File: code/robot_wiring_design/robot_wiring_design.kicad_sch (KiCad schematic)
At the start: 26 parts, among them J1 Conn_02x20_Counter_Clockwise

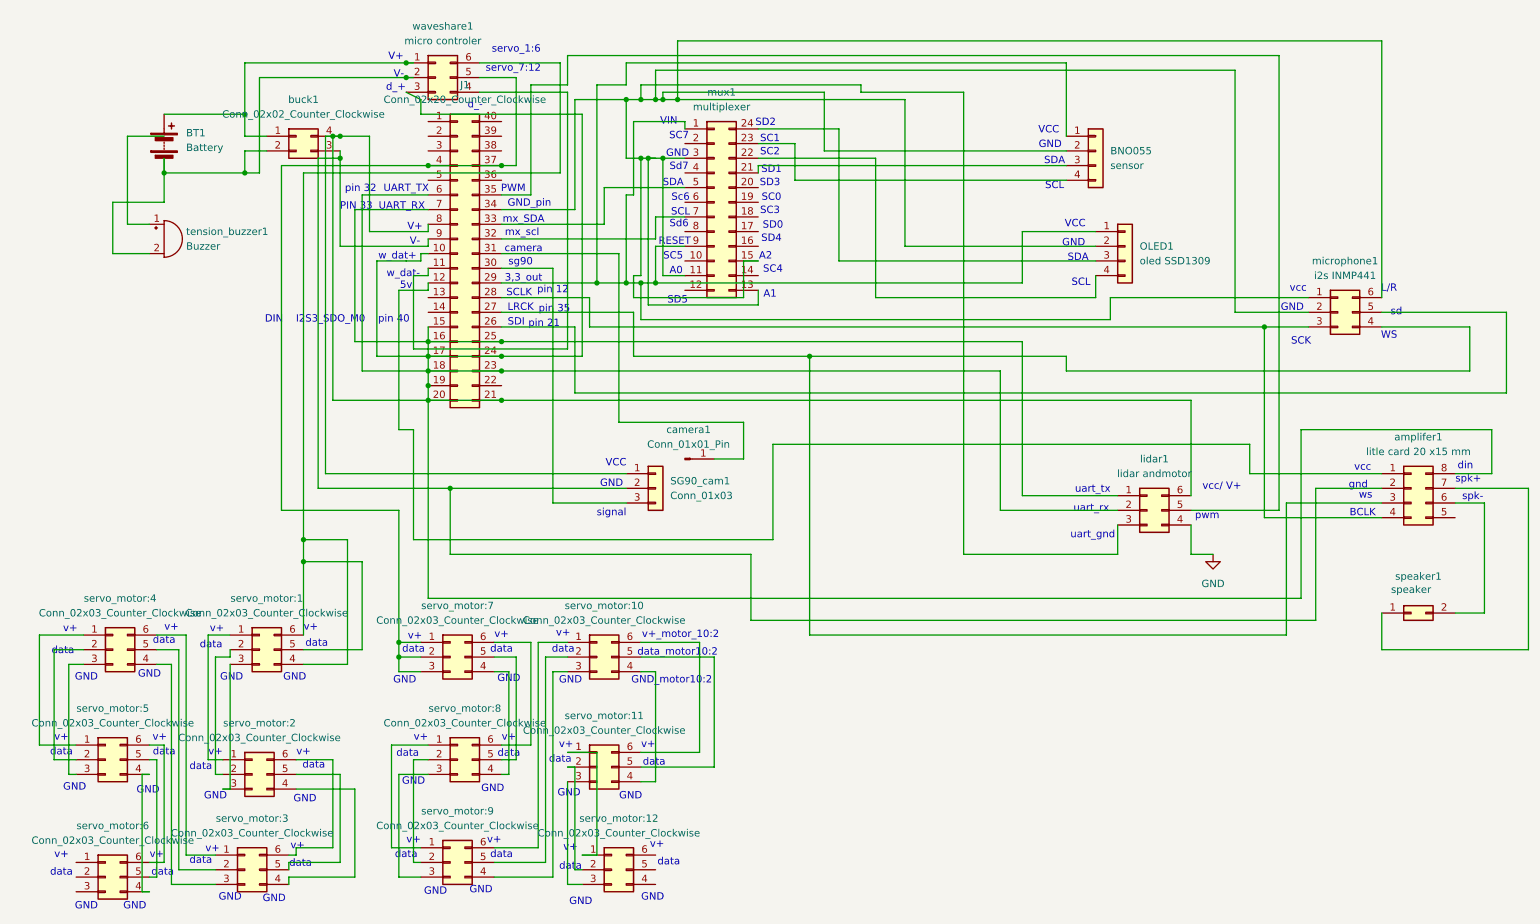
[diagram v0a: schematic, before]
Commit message: add the final pcb update the bom with lesspriced lidar add the new model of the 3d robot design
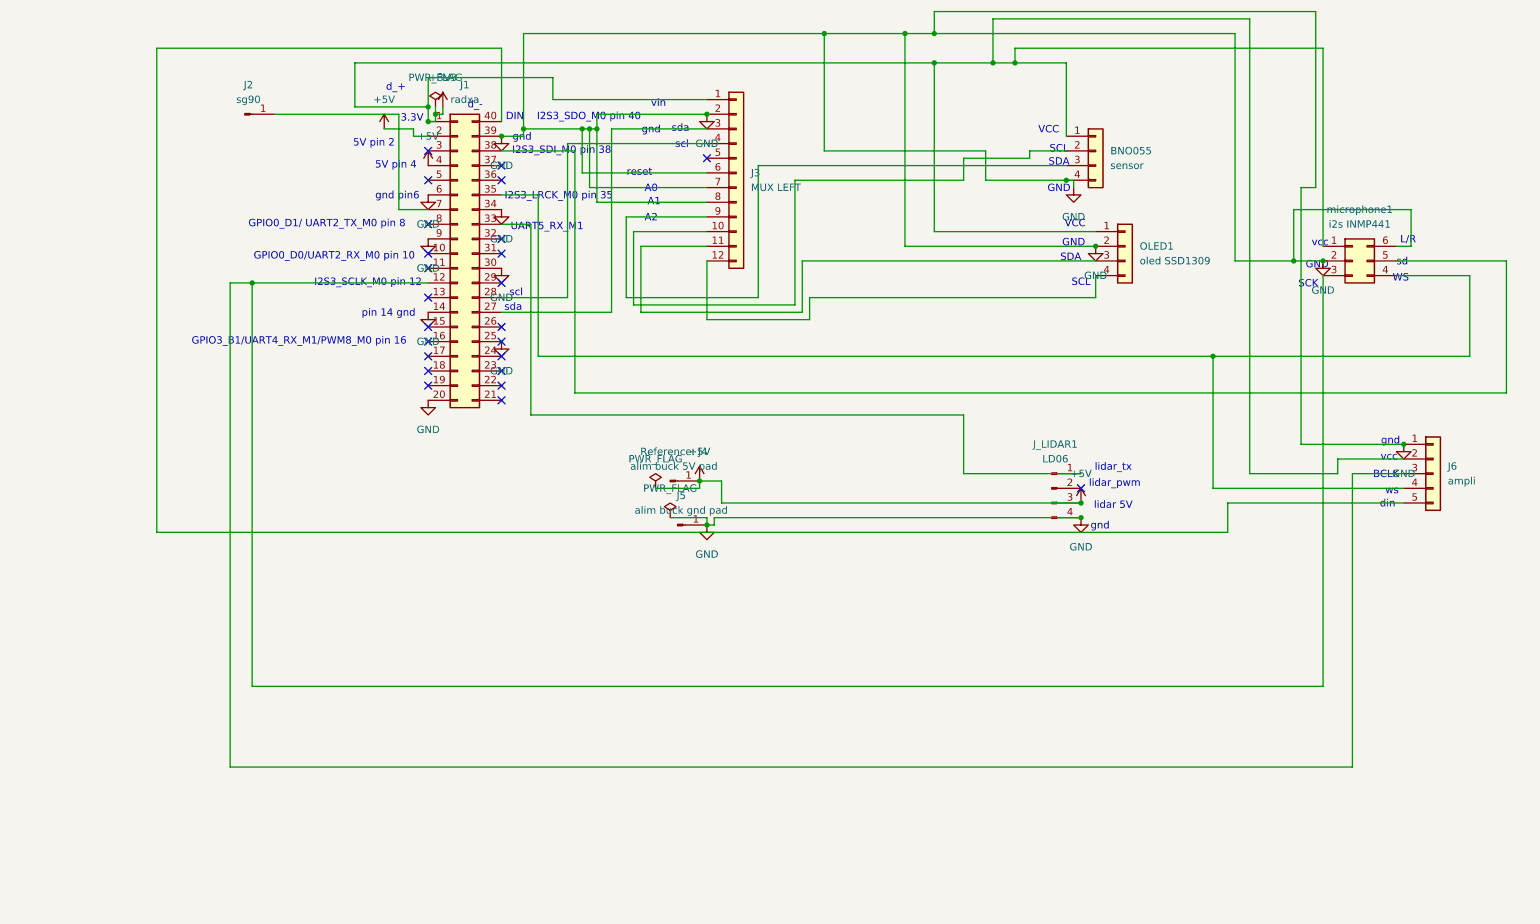
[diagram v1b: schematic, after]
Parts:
- removed BT1: Battery, symbol Device:Battery
- removed SG90_cam1: Conn_01x03, symbol Connector_Generic:Conn_01x03
- removed amplifer1: litle card 20 x15 mm, symbol Connector_Generic:Conn_02x04_Counter_Clockwise
- removed buck1: Conn_02x02_Counter_Clockwise, symbol Connector_Generic:Conn_02x02_Counter_Clockwise
- removed camera1: Conn_01x01_Pin, symbol Connector:Conn_01x01_Pin
- removed lidar1: lidar andmotor, symbol Connector_Generic:Conn_02x03_Counter_Clockwise
- removed mux1: multiplexer, Connector_PinHeader_2.54mm:PinHeader_2x12_P2.54mm_Vertical, symbol Connector_Generic:Conn_02x12_Counter_Clockwise
- removed servo_motor:1, servo_motor:10, servo_motor:11, servo_motor:12, servo_motor:2, servo_motor:3, servo_motor:4, servo_motor:5, servo_motor:6, servo_motor:7, servo_motor:8, servo_motor:9: Conn_02x03_Counter_Clockwise, symbol Connector_Generic:Conn_02x03_Counter_Clockwise
- removed speaker1: speaker, symbol Connector_Generic:Conn_02x01
- removed tension_buzzer1: Buzzer, symbol Device:Buzzer
- removed waveshare1: micro controler, symbol Connector_Generic:Conn_02x03_Counter_Clockwise
- added J2: sg90, Connector_Wire:SolderWirePad_1x01_SMD_5x10mm, symbol Connector:Conn_01x01_Pin
- added J3: MUX LEFT, Connector_PinHeader_2.54mm:PinHeader_1x12_P2.54mm_Vertical, symbol Connector_Generic:Conn_01x12
- added J4: alim buck 5V pad, Connector_Wire:SolderWirePad_1x01_SMD_5x10mm, symbol Connector:Conn_01x01_Pin
- added J5: alim buck gnd pad, Connector_Wire:SolderWirePad_1x01_SMD_5x10mm, symbol Connector:Conn_01x01_Pin
- added J6: ampli, TerminalBlock:TerminalBlock_MaiXu_MX126-5.0-05P_1x05_P5.00mm, symbol Connector_Generic:Conn_01x05
- added J_LIDAR1: LD06, TerminalBlock:TerminalBlock_MaiXu_MX126-5.0-04P_1x04_P5.00mm, symbol Connector:Conn_01x04_Pin
- J1: value Conn_02x20_Counter_Clockwise -> radxa
- OLED1: footprint Connector_PinHeader_2.54mm:PinHeader_1x04_P2.54mm_Vertical -> TerminalBlock:TerminalBlock_MaiXu_MX126-5.0-04P_1x04_P5.00mm
- microphone1: footprint (none) -> TerminalBlock:TerminalBlock_MaiXu_MX126-5.0-06P_1x06_P5.00mm
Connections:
- net GND: now also BNO055.4 (Pin_4), J1.14 (Pin_14), J1.20 (Pin_20), J1.25 (Pin_25), J1.30 (Pin_30), J1.34 (Pin_34), J1.39 (Pin_39), J1.6 (Pin_6), J1.9 (Pin_9), OLED1.2 (Pin_2), microphone1.2 (Pin_2), microphone1.6 (Pin_6), J3.2 (Pin_2), J3.6 (Pin_6), J3.7 (Pin_7), J3.8 (Pin_8), J5.1 (Pin_1), J6.1 (Pin_1), J_LIDAR1.4 (Pin_4)
- net at J1.35 (Pin_35): now also microphone1.4 (Pin_4), J6.4 (Pin_4)
- net +3V3: now reaches J1.1 (Pin_1)
- net +3V3: now also BNO055.1 (Pin_1), OLED1.1 (Pin_1), microphone1.1 (Pin_1), J3.1 (Pin_1), J6.2 (Pin_2)
- net at J1.12 (Pin_12): now also microphone1.3 (Pin_3), J6.3 (Pin_3)
- net +5V: now reaches J1.2 (Pin_2)
- net +5V: now also J1.4 (Pin_4), J4.1 (Pin_1), J_LIDAR1.3 (Pin_3)
- net at J1.26 (Pin_26): no longer microphone1.5 (Pin_5)
- net at J1.27 (Pin_27): now also J3.3 (Pin_3); no longer microphone1.4 (Pin_4)
- net at J1.28 (Pin_28): now also J3.4 (Pin_4); no longer microphone1.3 (Pin_3)
- net at J1.33 (Pin_33): now also J_LIDAR1.1 (Pin_1)
- net at J1.37 (Pin_37): no longer J1.4 (Pin_4)
- net at J1.38 (Pin_38): now also microphone1.5 (Pin_5)
- net at J1.40 (Pin_40): now also J6.5 (Pin_5)
- net at OLED1.3 (Pin_3): now also J3.11 (Pin_11)
- net at OLED1.4 (Pin_4): now also J3.12 (Pin_12)
- net at BNO055.3 (Pin_3): now also J3.9 (Pin_9)
- new net: J1.7 (Pin_7), J2.1 (Pin_1)
- new net: BNO055.2 (Pin_2), J3.10 (Pin_10)
- now unconnected: J1.10 (Pin_10), J1.15 (Pin_15), J1.16 (Pin_16), J1.17 (Pin_17), J1.18 (Pin_18), J1.19 (Pin_19), J1.21 (Pin_21), J1.23 (Pin_23), J1.24 (Pin_24), J1.29 (Pin_29), J1.8 (Pin_8)
- no-connect marks 0 -> 24
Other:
- note added: "3.3V"
- note added: "5V pin 2"
- note added: "5V pin 4"
- note added: "GPIO0_D0/UART2_RX_M0 pin 10"
- note added: "GPIO0_D1/ UART2_TX_M0 pin 8"
- note added: "GPIO3_B1/UART4_RX_M1/PWM8_M0 pin 16"
- note added: "I2S3_LRCK_M0 pin 35"
- note added: "I2S3_SCLK_M0 pin 12"
- note added: "I2S3_SDI_M0 pin 38"
- note added: "UART5_RX_M1"
- note added: "gnd pin6"
- note added: "lidar 5V"
- note added: "lidar_pwm"
- note added: "lidar_tx"
- note added: "pin 14 gnd"
- note added: "reset"
- note added: "scl"
- note added: "sda"
- note added: "vin"
- note removed: "3,3_out"
- note removed: "5v"
- note removed: "GND_motor10:2"
- note removed: "GND_pin"
- note removed: "LRCK"
- note removed: "PIN 33"
- note removed: "PWM"
- note removed: "RESET"
- note removed: "SC0"
- note removed: "SC1"
- note removed: "SC2"
- note removed: "SC3"
- note removed: "SC4"
- note removed: "SC5"
- note removed: "SC7"
- note removed: "SCLK"
- note removed: "SD0"
- note removed: "SD1"
- note removed: "SD2"
- note removed: "SD3"
- note removed: "SD4"
- note removed: "SD5"
- note removed: "SDI"
- note removed: "Sc6"
- note removed: "Sd6"
- note removed: "Sd7"
- note removed: "UART_RX"
- note removed: "UART_TX"
- note removed: "V+"
- note removed: "V-"
- note removed: "VIN"
- note removed: "camera"
- note removed: "data"
- note removed: "data_motor10:2"
- note removed: "mx_SDA"
- note removed: "mx_scl"
- note removed: "pin 12"
- note removed: "pin 21"
- note removed: "pin 32"
- note removed: "pin 35"
- note removed: "pwm"
- note removed: "servo_1:6"
- note removed: "servo_7:12"
- note removed: "sg90"
- note removed: "signal"
- note removed: "spk+"
- note removed: "spk-"
- note removed: "uart_gnd"
- note removed: "uart_rx"
- note removed: "uart_tx"
- note removed: "v+"
- note removed: "v+_motor_10:2"
- note removed: "vcc/ V+"
- note removed: "w_dat+"
- note removed: "w_dat-"
- moved on the sheet: microphone1
